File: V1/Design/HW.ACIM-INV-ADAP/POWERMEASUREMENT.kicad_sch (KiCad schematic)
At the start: 42 parts, among them U15 ISO OPAMP 1-CH, U17 OP-1CH, U18 OP-1CH, U19 OP-1CH, U2 OP-1CH

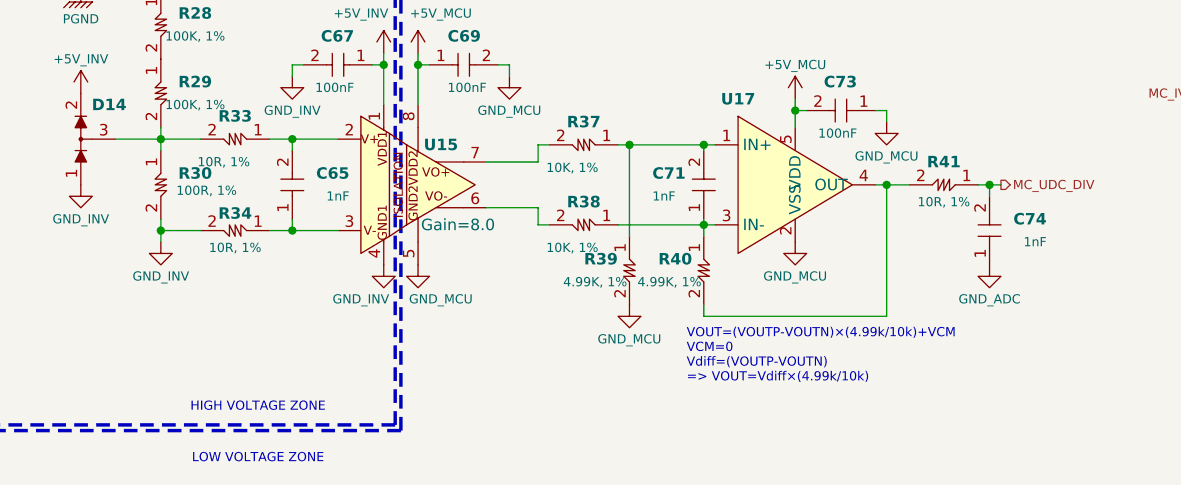
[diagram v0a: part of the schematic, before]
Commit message: HW.ACIM-ADAP schematic
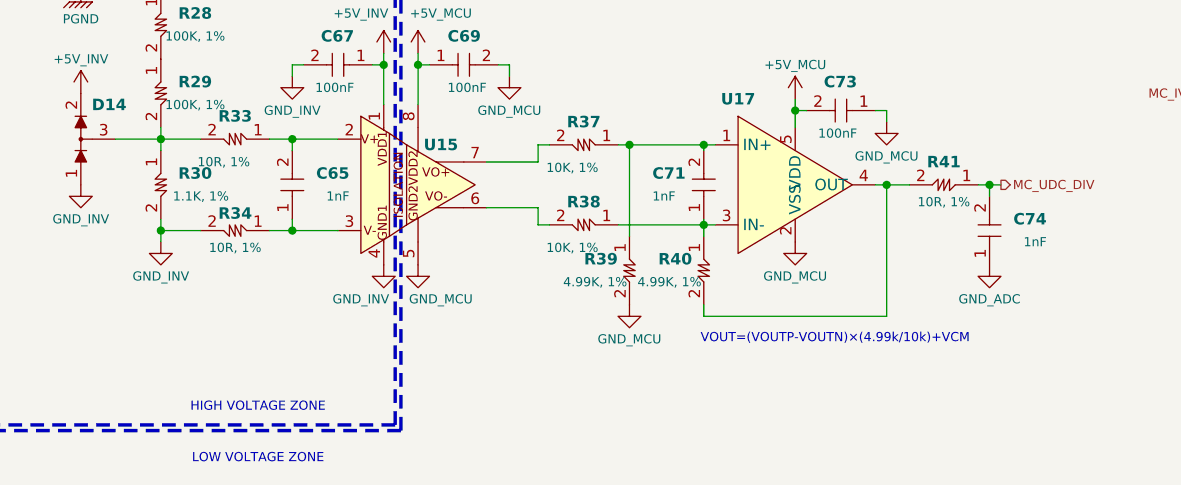
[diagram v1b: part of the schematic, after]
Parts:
- R30: value 100R, 1% -> 1.1K, 1%; MNP RC0603FR-07100RL -> RC0603FR-071K1L
- U15: Note Gain=8.0 -> (none)
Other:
- note added: "VOUT=(VOUTP-VOUTN)×(4.99k/10k)+VCM"
- note removed: "VOUT=(VOUTP-VOUTN)×(4.99k/10k)+VCM VCM=0 Vdiff=(VOUTP-VOUTN) => VOUT=Vdiff×(4.99k/10k)"
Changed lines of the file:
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@@
 		)
 	)
-	(text "VOUT=(VOUTP-VOUTN)×(4.99k/10k)+VCM\nVCM=0\nVdiff=(VOUTP-VOUTN)\n=> VOUT=Vdiff×(4.99k/10k)"
+	(text "VOUT=(VOUTP-VOUTN)×(4.99k/10k)+VCM"
 		(exclude_from_sim no)
-		(at 97.155 106.68 0)
+		(at 113.665 104.775 0)
 		(effects
 			(font
@@
 				(thickness 0.127)
 			)
-			(justify left)
 		)
 	)
@@
 			)
 		)
-		(property "Value" "100R, 1%"
-			(at 43.815 88.265 90)
+		(property "Value" "1.1K, 1%"
+			(at 43.18 88.9 90)
 			(effects
 				(font
@@
 			)
 		)
-		(property "Description" "RES 100R OHM 1% 1/10W 0603"
+		(property "Description" "RES 1.1K OHM 1% 1/10W 0603"
 			(at 36.195 86.36 0)
 			(effects
@@
 			)
 		)
-		(property "MNP" "RC0603FR-07100RL"
+		(property "MNP" "RC0603FR-071K1L"
 			(at 36.195 86.36 0)
 			(effects
@@
 			)
 		)
-		(property "Note" "Gain=8.0"
-			(at 71.755 92.075 0)
-			(effects
-				(font
-					(size 1.27 1.27)
-				)
-			)
-		)
